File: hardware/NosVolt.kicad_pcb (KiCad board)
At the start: 4 copper layers, 145 x 60 mm, 101 parts, among them CN201 100nF, J101 INPUTS, J102 OUTPUTS, J201 BAT_SENSE, J202 BAT_NTC, J401 USB_C_Receptacle_USB2.0_16P, Q1101 2N7002, Q1102 AO4407A, Q801 2N7002, Q802 AO4407A, Q901 2N7002, Q902 AO4407A, SW101 SW_Reset, SW102 SSSS811101, U1001 INA226, U101 ESP32-S3-WROOM-1, U102 GMT028-05, U1201 INA226, U201 ADS1115IDGS, U301 MP2307DN-LF-Z, U401 AP7361-33ER-13, U402 USBLC6-2SC6, U501 INA226, U601 INA226, U701 INA226

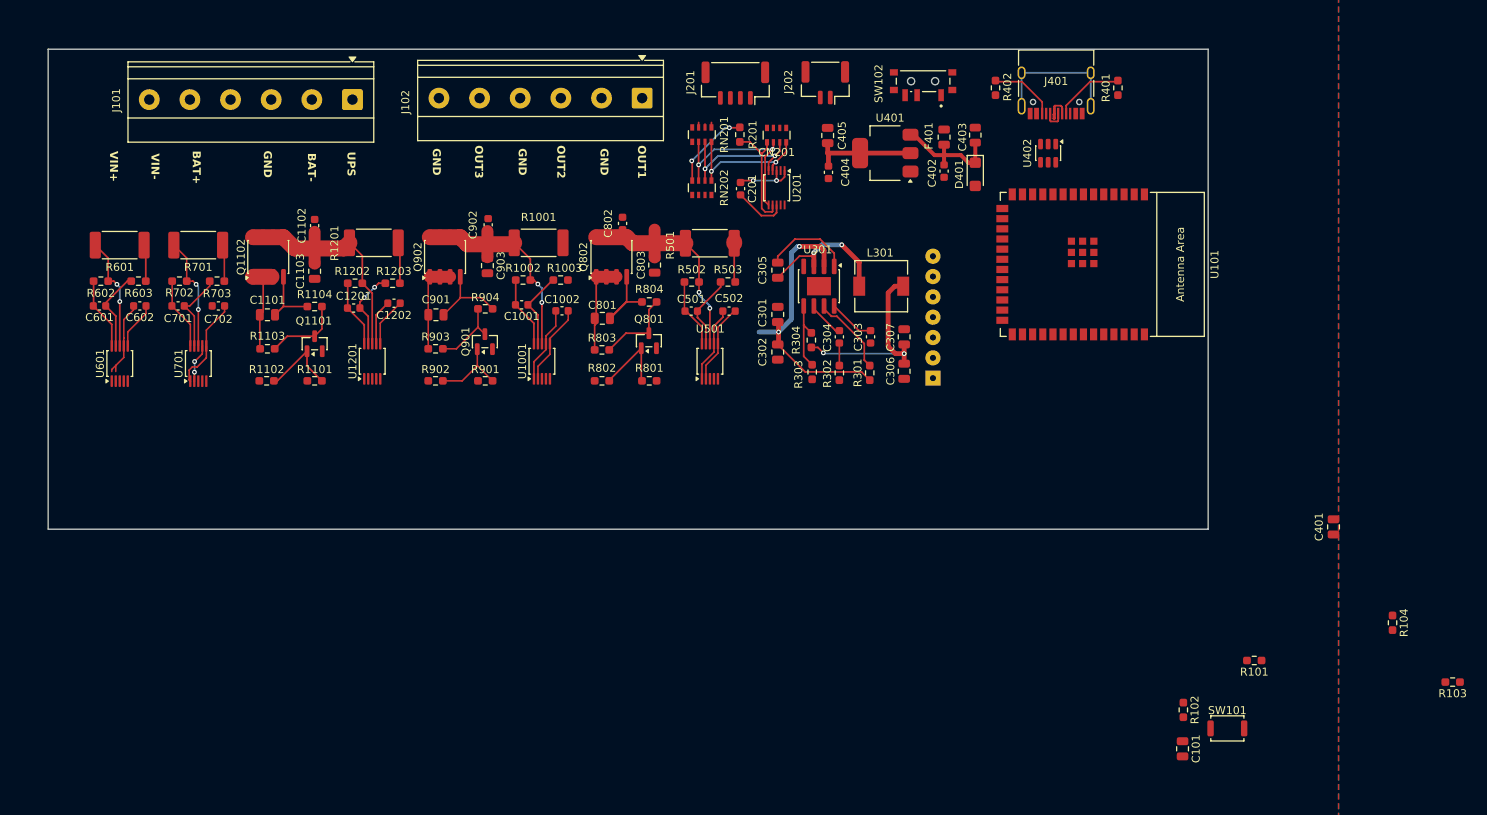
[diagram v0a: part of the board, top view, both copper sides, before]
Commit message: rc
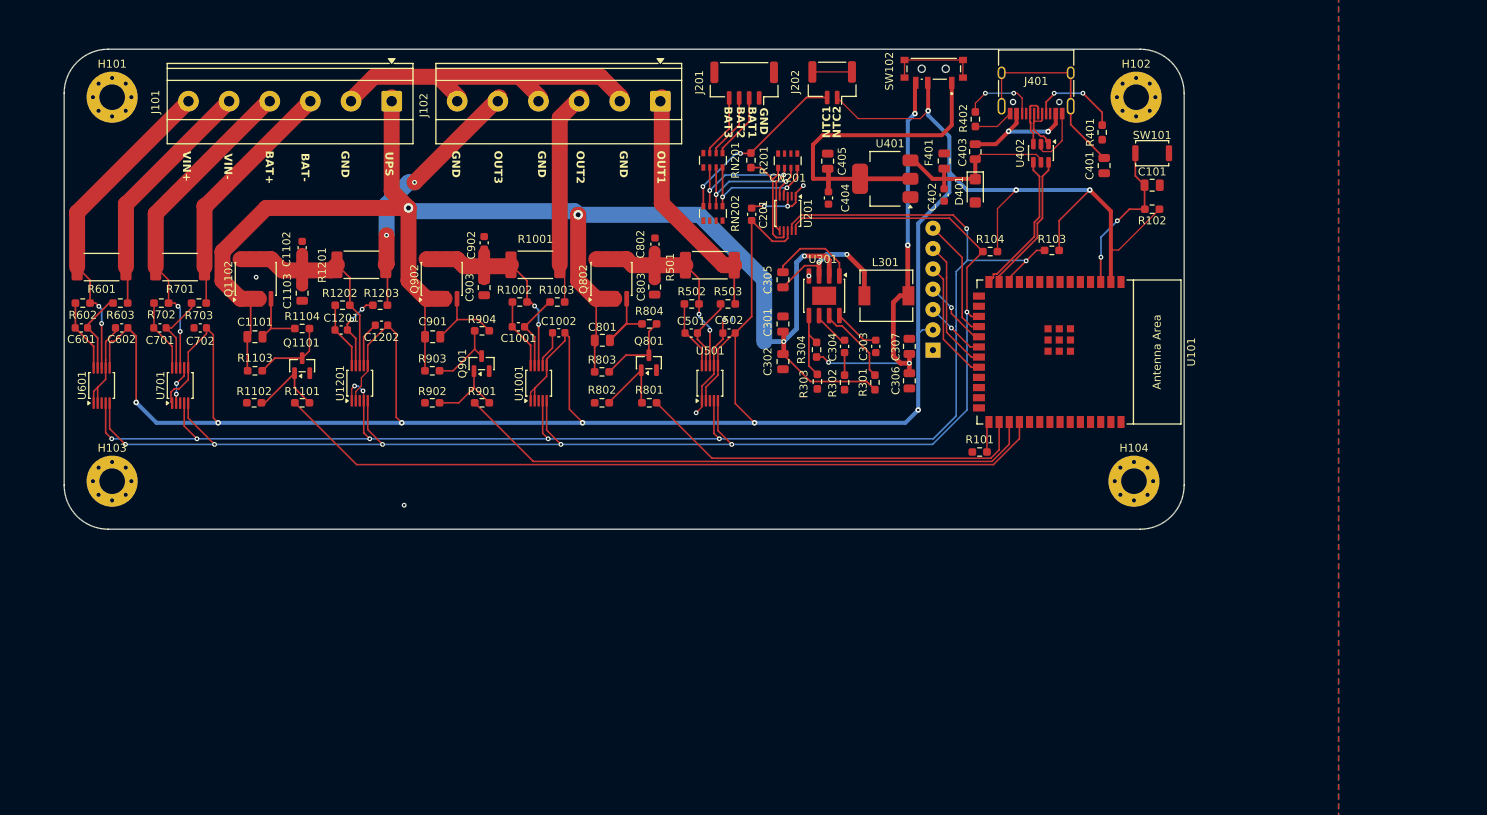
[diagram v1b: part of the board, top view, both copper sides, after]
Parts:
- added H101: MountingHole, MountingHole:MountingHole_3.2mm_M3_Pad_Via, F.Cu at (108.7, 43.8)
- added H102: MountingHole, MountingHole:MountingHole_3.2mm_M3_Pad_Via, F.Cu at (236.7, 43.8)
- added H103: MountingHole, MountingHole:MountingHole_3.2mm_M3_Pad_Via, F.Cu at (108.7, 91.8)
- added H104: MountingHole, MountingHole:MountingHole_3.2mm_M3_Pad_Via, F.Cu at (236.4, 91.8)
- moved R103 73.6 mm to (226.2, 63.0)
- moved SW101 72.5 mm to (238.7, 50.8)
- moved C101 70.6 mm to (238.7, 54.8), turned to 0 degrees
- moved R104 68.4 mm to (218.4, 63.1), turned to 180 degrees
- moved R102 62.7 mm to (238.7, 57.8), turned to 180 degrees
- moved C401 53.5 mm to (232.7, 52.4)
- moved R101 43.1 mm to (217.1, 88.2)
- moved U101 11.3 mm to (226.6, 75.7)
- moved R401 5.91 mm to (232.4, 48.2)
- moved J101 4.90 mm to (143.6, 44.3)
- moved C802 4.81 mm to (176.6, 62.2)
- moved R402 4.66 mm to (216.6, 46.5)
- moved C601 3.56 mm to (104.9, 72.6)
- moved C602 3.56 mm to (109.9, 72.6)
- moved C701 3.56 mm to (114.7, 72.6)
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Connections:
- SW102 pad 1: unconnected-(SW102-Pad1) -> /USB_LDO/USB_3V3
- U101 pad 28: unconnected-(U101-SPIIO6/GPIO35/FSPID/SUBSPID-Pad28) -> EN_OUT1
- U101 pad 29: unconnected-(U101-SPIIO7/GPIO36/FSPICLK/SUBSPICLK-Pad29) -> EN_OUT2
- U101 pad 30: unconnected-(U101-SPIDQS/GPIO37/FSPIQ/SUBSPIQ-Pad30) -> EN_OUT3
- U101 pad 4: EN_OUT1 -> unconnected-(U101-GPIO4/TOUCH4/ADC1_CH3-Pad4)
- U101 pad 5: EN_OUT2 -> unconnected-(U101-GPIO5/TOUCH5/ADC1_CH4-Pad5)
- U101 pad 6: EN_OUT3 -> unconnected-(U101-GPIO6/TOUCH6/ADC1_CH5-Pad6)
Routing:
- net +3.3V: track 50.8 -> 347.6 mm, vias 0 -> 9
- net SDA: track 0.00 -> 198.1 mm, vias 0 -> 9
- net SCL: track 0.00 -> 186.6 mm, vias 0 -> 6
- net +12V_UPS: track 70.6 -> 196.7 mm, vias 2 -> 4
- net EN_OUT3: track 0.00 -> 97.2 mm
- net GND: track 47.5 -> 123.1 mm, vias 4 -> 10
- net EN_OUT2: track 0.00 -> 73.5 mm
- net EN_OUT1: track 0.00 -> 49.6 mm
- net /USB_LDO/USB_3V3: track 13.3 -> 43.1 mm
- net /Output3/VOUT: track 5.14 -> 32.4 mm, vias 0 -> 2
- net /MP2307/OUT: track 25.6 -> 52.7 mm, vias 2 -> 4
- net /Output2/VOUT: track 0.00 -> 26.9 mm
- net /INA226_BAT/VIN: track 14.3 -> 41.1 mm
- net /INA226_IN/VIN: track 14.3 -> 40.8 mm
- net /INA226_BAT/VOUT: track 4.29 -> 30.7 mm
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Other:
- board size 145 x 60 mm -> 140 x 60 mm
- board text added: "BAT1"
- board text added: "BAT2"
- board text added: "BAT3"
- board text added: "NTC1"
- board text added: "NTC2"

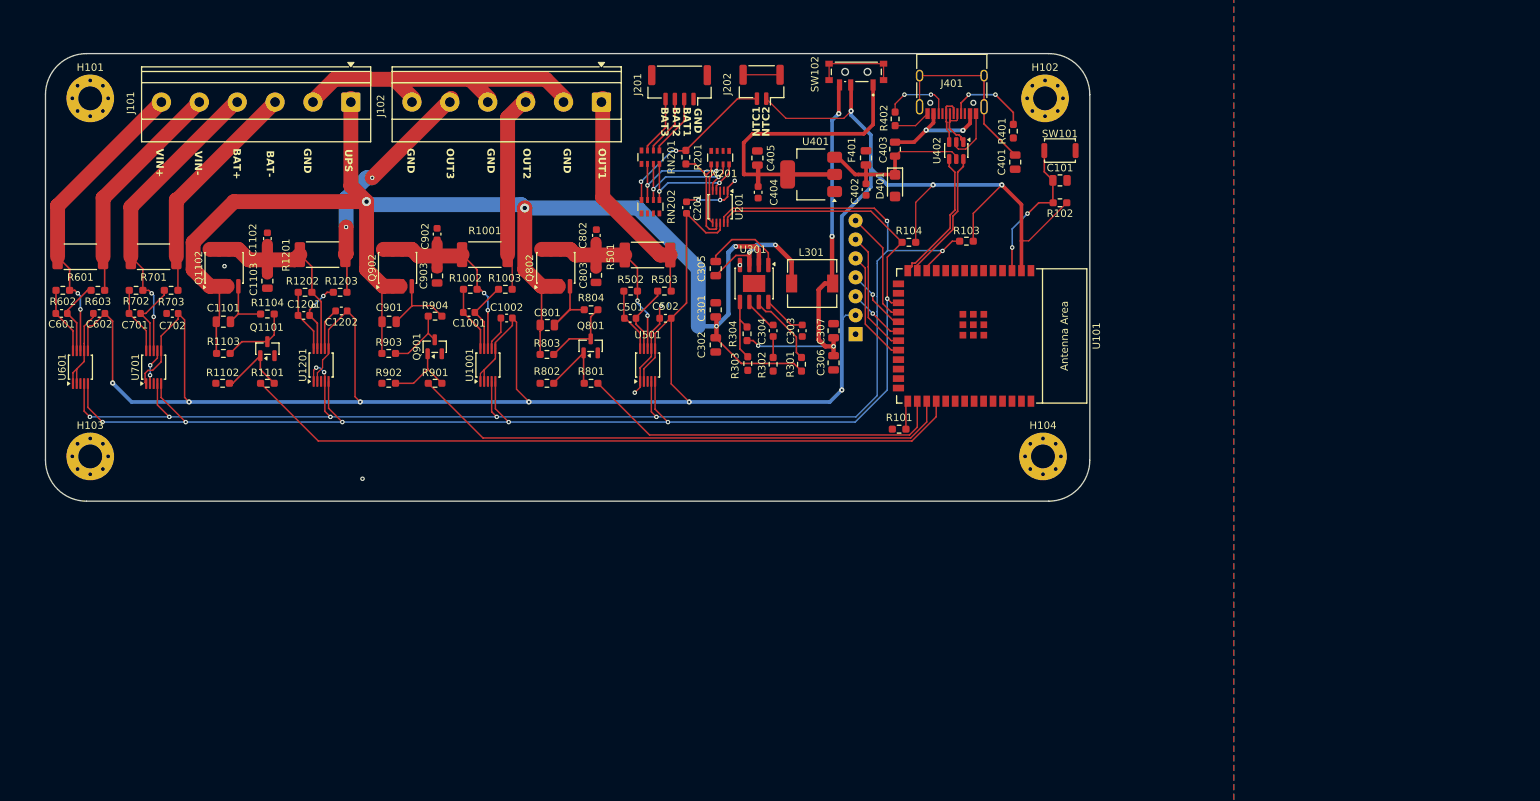
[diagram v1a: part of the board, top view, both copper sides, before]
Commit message: 100*100
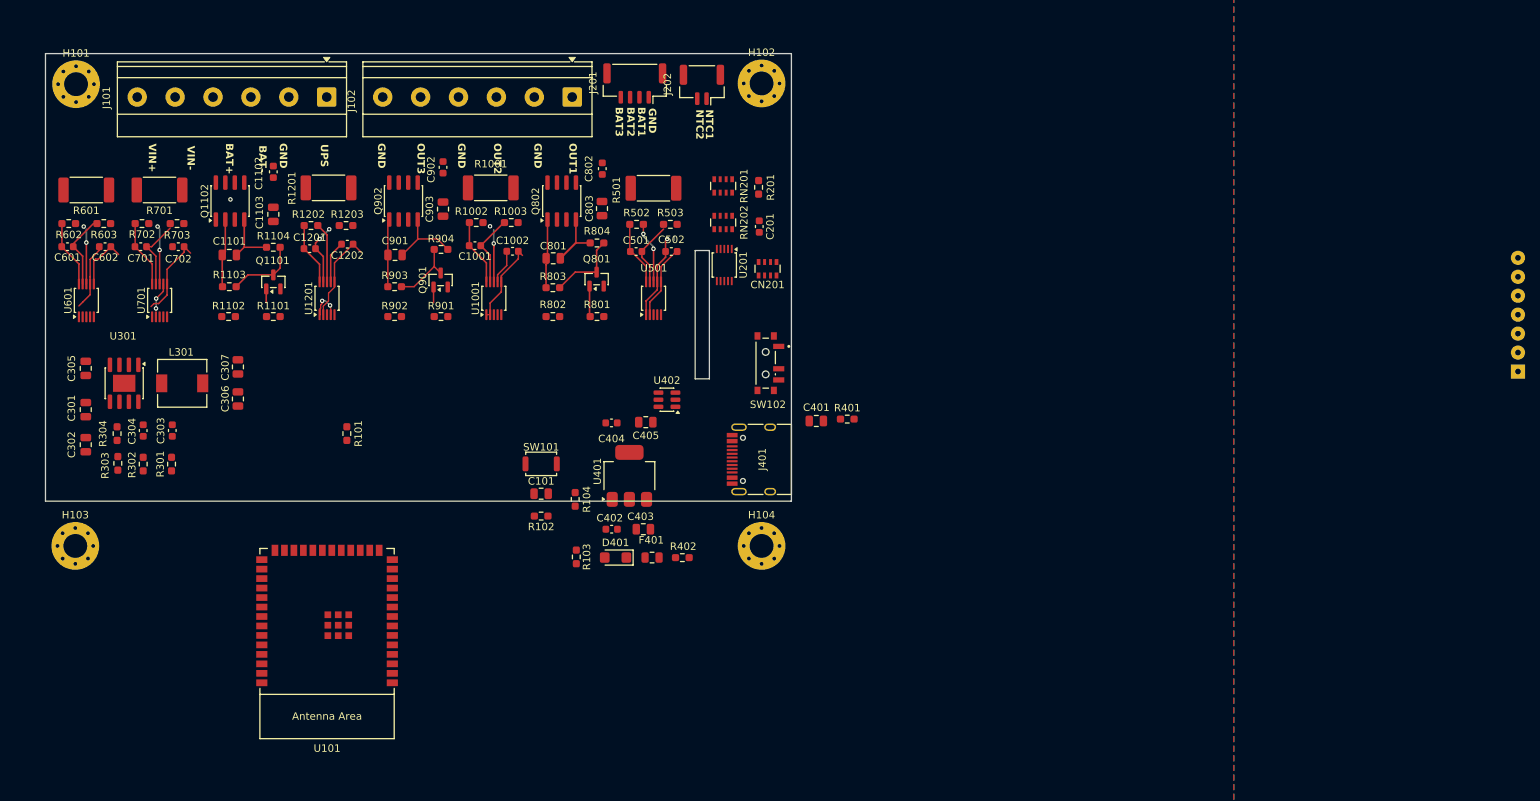
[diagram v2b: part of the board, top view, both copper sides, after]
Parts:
- moved U101 94.2 mm to (140.4, 113.9), turned to 180 degrees
- moved U102 88.9 mm to (262.0, 72.8)
- moved C301 85.5 mm to (108.1, 85.5)
- moved C302 85.5 mm to (108.1, 90.2)
- moved C305 85.5 mm to (108.1, 80.0)
- moved R301 85.5 mm to (119.6, 92.8)
- moved C303 85.5 mm to (119.7, 88.3)
- moved C304 85.5 mm to (115.8, 88.3)
- moved R302 85.5 mm to (115.8, 92.8)
- moved R304 85.5 mm to (112.3, 88.7)
- moved L301 85.5 mm to (121.0, 82.0)
- moved R303 85.5 mm to (112.4, 92.7)
- moved U301 85.5 mm to (113.2, 82.0)
- moved C101 81.2 mm to (169.2, 96.8)
- moved R102 81.2 mm to (169.2, 99.8)
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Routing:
- net +3.3V: track 347.6 -> 53.4 mm, vias 9 -> 0
- net SDA: track 198.1 -> 4.63 mm, vias 9 -> 2
- net SCL: track 186.6 -> 0.00 mm, vias 6 -> 0
- net +12V_UPS: track 196.7 -> 26.5 mm, vias 4 -> 0
- net EN_OUT3: track 97.2 -> 0.00 mm
- net GND: track 123.1 -> 34.8 mm, vias 10 -> 4
- net EN_OUT2: track 73.5 -> 0.00 mm
- net /MP2307/OUT: track 52.7 -> 0.00 mm, vias 4 -> 0
- net EN_OUT1: track 49.6 -> 0.00 mm
- net /USB_LDO/USB_3V3: track 43.1 -> 0.00 mm
- net /INA226_BAT/VIN: track 41.1 -> 7.43 mm
- net /INA226_IN/VIN: track 40.8 -> 7.35 mm
- net /Output3/VOUT: track 32.4 -> 0.00 mm, vias 2 -> 0
- net /INA226_BAT/VOUT: track 30.7 -> 0.00 mm
- net /Output1/VOUT: track 30.5 -> 0.00 mm
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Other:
- board size 140 x 60 mm -> 100 x 60 mm
